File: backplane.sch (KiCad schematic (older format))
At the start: 29 parts, among them J1 I2C, J2 I2C, J3 SER, J4 PWR, J5 PWR, J6 FAN, Q1 Q_NMOS_GSD, Q2 Q_NMOS_GSD, Q3 Q_NMOS_GSD, Q4 Q_NMOS_GSD, U1 Raspberry_Pi_2_3, U2 IC880A-SPI, U3 SHT21, U4 MP1584_MODULE

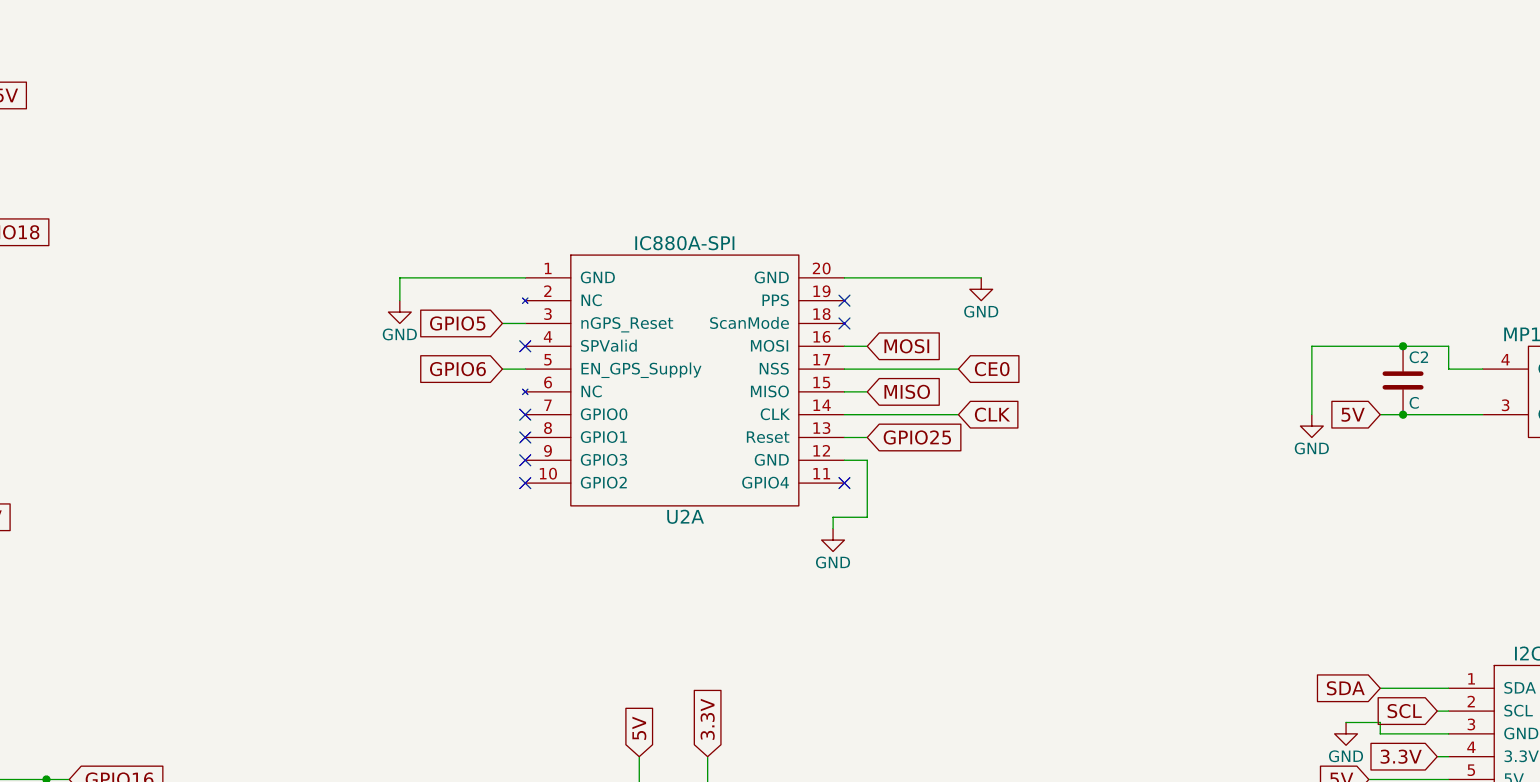
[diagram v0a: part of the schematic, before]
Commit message: Add ADC (refs #14)
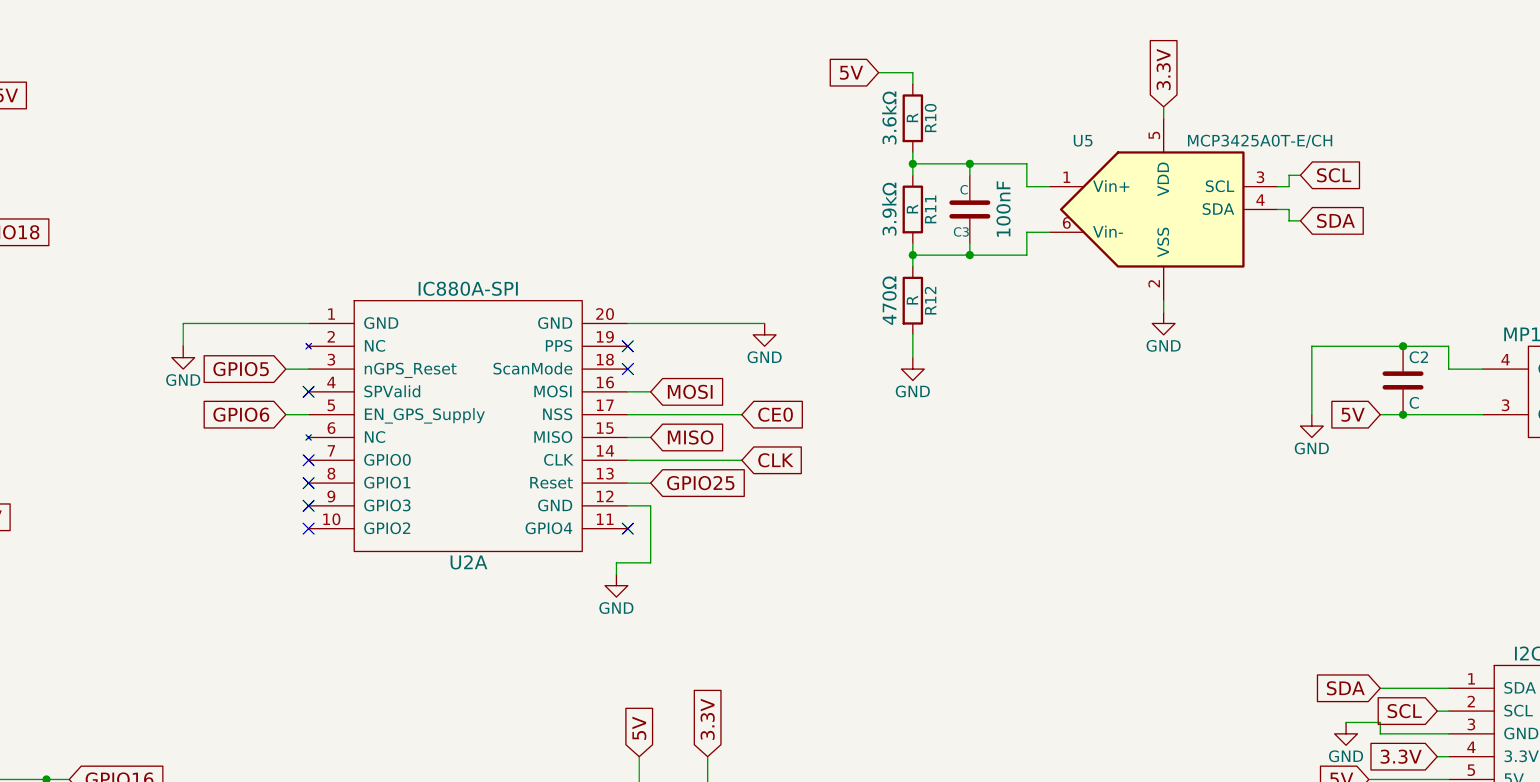
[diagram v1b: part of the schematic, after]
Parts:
- added C3: C, Capacitors_SMD:C_1206, symbol C
- added R10, R11, R12: R, symbol R
- added U5: MCP3425A0T-E/CH, symbol MCP3425A0T-E/CH
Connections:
- net 3.3V: now also U5.5 (VDD)
- net 5V: now also R10.1
- net GND: now also R12.2, U5.2 (VSS)
- net SCL: now also U5.3 (SCL)
- net SDA: now also U5.4 (SDA)
- new net: C3.2, R10.2, R11.1, U5.1 (Vin+)
- new net: C3.1, R11.2, R12.1, U5.6 (Vin-)
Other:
- moved on the sheet: U2A

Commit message: Assign footprints to ADC (refs #14)
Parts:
- R10, R11, R12: footprint (none) -> Resistors_SMD:R_0805_HandSoldering
- U5: footprint (none) -> TO_SOT_Packages_SMD:SOT-23-6_Handsoldering
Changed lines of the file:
@@
 $EndComp
 $Comp
-L GND-RESCUE-backplane #PWR13
+L GND-RESCUE-backplane #PWR01
 U 1 1 58965F26
 P 1650 4000
-F 0 "#PWR13" H 1650 3750 50  0001 C CNN
+F 0 "#PWR01" H 1650 3750 50  0001 C CNN
 F 1 "GND" H 1650 3850 50  0000 C CNN
 F 2 "" H 1650 4000 50  0000 C CNN
@@
 $EndComp
 $Comp
-L GND-RESCUE-backplane #PWR17
+L GND-RESCUE-backplane #PWR02
 U 1 1 58965F7C
 P 850 5000
-F 0 "#PWR17" H 850 4750 50  0001 C CNN
+F 0 "#PWR02" H 850 4750 50  0001 C CNN
 F 1 "GND" H 850 4850 50  0000 C CNN
 F 2 "" H 850 5000 50  0000 C CNN
@@
 $EndComp
 $Comp
-L GND-RESCUE-backplane #PWR15
+L GND-RESCUE-backplane #PWR03
 U 1 1 58965FBA
 P 1250 4500
-F 0 "#PWR15" H 1250 4250 50  0001 C CNN
+F 0 "#PWR03" H 1250 4250 50  0001 C CNN
 F 1 "GND" H 1250 4350 50  0000 C CNN
 F 2 "" H 1250 4500 50  0000 C CNN
@@
 $EndComp
 $Comp
-L GND-RESCUE-backplane #PWR21
+L GND-RESCUE-backplane #PWR04
 U 1 1 5896BA26
 P 4950 6850
-F 0 "#PWR21" H 4950 6600 50  0001 C CNN
+F 0 "#PWR04" H 4950 6600 50  0001 C CNN
 F 1 "GND" H 4950 6700 50  0000 C CNN
 F 2 "" H 4950 6850 50  0000 C CNN
@@
 $EndComp
 $Comp
-L GND-RESCUE-backplane #PWR3
+L GND-RESCUE-backplane #PWR05
 U 1 1 589714DC
 P 5750 1750
-F 0 "#PWR3" H 5750 1500 50  0001 C CNN
+F 0 "#PWR05" H 5750 1500 50  0001 C CNN
 F 1 "GND" H 5750 1600 50  0000 C CNN
 F 2 "" H 5750 1750 50  0000 C CNN
@@
 $EndComp
 $Comp
-L GND-RESCUE-backplane #PWR9
+L GND-RESCUE-backplane #PWR06
 U 1 1 589715AD
 P 5100 2850
-F 0 "#PWR9" H 5100 2600 50  0001 C CNN
+F 0 "#PWR06" H 5100 2600 50  0001 C CNN
 F 1 "GND" H 5100 2700 50  0000 C CNN
 F 2 "" H 5100 2850 50  0000 C CNN
@@
 $EndComp
 $Comp
-L GND-RESCUE-backplane #PWR6
+L GND-RESCUE-backplane #PWR07
 U 1 1 589716C7
 P 3200 1850
-F 0 "#PWR6" H 3200 1600 50  0001 C CNN
+F 0 "#PWR07" H 3200 1600 50  0001 C CNN
 F 1 "GND" H 3200 1700 50  0000 C CNN
 F 2 "" H 3200 1850 50  0000 C CNN
@@
 $EndComp
 $Comp
-L GND #PWR20
+L GND #PWR08
 U 1 1 5898B674
 P 2200 6400
-F 0 "#PWR20" H 2200 6400 30  0001 C CNN
+F 0 "#PWR08" H 2200 6400 30  0001 C CNN
 F 1 "GND" H 2200 6330 30  0001 C CNN
 F 2 "" H 2200 6400 60  0001 C CNN
@@
 F 1 "SHT21" H 9350 5300 60  0000 C CNN
 F 2 "sensirion:SHT21" H 9350 5000 60  0001 C CNN
-F 3 "" H 9350 5000 60  0001 C CNN
+F 3 "https://www.sensirion.com/fileadmin/user_upload/customers/sensirion/Dokumente/2_Humidity_Sensors/Sensirion_Humidity_Sensors_SHT21_Datasheet_V4.pdf" H 9350 5000 60  0001 C CNN
 	1    9350 5000
 	1    0    0    -1
@@
 F 1 "C" H 9356 4415 40  0000 L CNN
 F 2 "Capacitors_SMD:C_1206" H 9388 4350 30  0001 C CNN
-F 3 "https://www.sensirion.com/fileadmin/user_upload/customers/sensirion/Dokumente/2_Humidity_Sensors/Sensirion_Humidity_Sensors_SHT21_Datasheet_V4.pdf" H 9350 4500 60  0001 C CNN
+F 3 "" H 9350 4500 60  0001 C CNN
 F 4 "100nF" V 9200 4500 60  0000 C CNN "C"
 	1    9350 4500
@@
 $EndComp
 $Comp
-L GND #PWR12
+L GND #PWR09
 U 1 1 58A239AE
 P 2200 3950
-F 0 "#PWR12" H 2200 3700 50  0001 C CNN
+F 0 "#PWR09" H 2200 3700 50  0001 C CNN
 F 1 "GND" H 2200 3800 50  0000 C CNN
 F 2 "" H 2200 3950 50  0000 C CNN
@@
 $EndComp
 $Comp
-L GND #PWR14
+L GND #PWR010
 U 1 1 58A23A76
 P 2200 4450
-F 0 "#PWR14" H 2200 4200 50  0001 C CNN
+F 0 "#PWR010" H 2200 4200 50  0001 C CNN
 F 1 "GND" H 2200 4300 50  0000 C CNN
 F 2 "" H 2200 4450 50  0000 C CNN
@@
 $EndComp
 $Comp
-L GND #PWR16
+L GND #PWR011
 U 1 1 58A23B3E
 P 2200 4950
-F 0 "#PWR16" H 2200 4700 50  0001 C CNN
+F 0 "#PWR011" H 2200 4700 50  0001 C CNN
 F 1 "GND" H 2200 4800 50  0000 C CNN
 F 2 "" H 2200 4950 50  0000 C CNN
@@
 $EndComp
 $Comp
-L GND #PWR5
+L GND #PWR012
 U 1 1 58A90AD5
 P 2000 1850
-F 0 "#PWR5" H 2000 1600 50  0001 C CNN
+F 0 "#PWR012" H 2000 1600 50  0001 C CNN
 F 1 "GND" H 2000 1700 50  0000 C CNN
 F 2 "" H 2000 1850 50  0000 C CNN
@@
 5V
 $Comp
-L GND #PWR4
+L GND #PWR013
 U 1 1 58F15EFB
 P 1600 1850
-F 0 "#PWR4" H 1600 1600 50  0001 C CNN
+F 0 "#PWR013" H 1600 1600 50  0001 C CNN
 F 1 "GND" H 1600 1700 50  0000 C CNN
 F 2 "" H 1600 1850 50  0000 C CNN
@@
 $EndComp
 $Comp
-L GND #PWR8
+L GND #PWR014
 U 1 1 58F163DE
 P 8150 2150
-F 0 "#PWR8" H 8150 1900 50  0001 C CNN
+F 0 "#PWR014" H 8150 1900 50  0001 C CNN
 F 1 "GND" H 8150 2000 50  0000 C CNN
 F 2 "" H 8150 2150 50  0000 C CNN
@@
 5V
 $Comp
-L GND #PWR1
+L GND #PWR015
 U 1 1 58F16888
 P 9750 1350
-F 0 "#PWR1" H 9750 1100 50  0001 C CNN
+F 0 "#PWR015" H 9750 1100 50  0001 C CNN
 F 1 "GND" H 9750 1200 50  0000 C CNN
 F 2 "" H 9750 1350 50  0000 C CNN
@@
 GPIO18
 $Comp
-L GND #PWR19
+L GND #PWR016
 U 1 1 58F17ECB
 P 3750 6250
-F 0 "#PWR19" H 3750 6000 50  0001 C CNN
+F 0 "#PWR016" H 3750 6000 50  0001 C CNN
 F 1 "GND" H 3750 6100 50  0000 C CNN
 F 2 "" H 3750 6250 50  0000 C CNN
@@
 5V
 $Comp
-L PWR_FLAG #FLG1
+L PWR_FLAG #FLG017
 U 1 1 58F18E09
 P 3750 6150
-F 0 "#FLG1" H 3750 6245 50  0001 C CNN
+F 0 "#FLG017" H 3750 6245 50  0001 C CNN
 F 1 "PWR_FLAG" H 3750 6330 50  0000 C CNN
 F 2 "" H 3750 6150 50  0000 C CNN
@@
 SDA
 $Comp
-L GND #PWR11
+L GND #PWR018
 U 1 1 58F1F392
 P 9600 3500
-F 0 "#PWR11" H 9600 3250 50  0001 C CNN
+F 0 "#PWR018" H 9600 3250 50  0001 C CNN
 F 1 "GND" H 9600 3350 50  0000 C CNN
 F 2 "" H 9600 3500 50  0000 C CNN
@@
 SDA
 $Comp
-L GND #PWR10
+L GND #PWR019
 U 1 1 58F20596
 P 8300 3500
-F 0 "#PWR10" H 8300 3250 50  0001 C CNN
+F 0 "#PWR019" H 8300 3250 50  0001 C CNN
 F 1 "GND" H 8300 3350 50  0000 C CNN
 F 2 "" H 8300 3500 50  0000 C CNN
@@
 3.3V
 $Comp
-L GND #PWR18
+L GND #PWR020
 U 1 1 58F2395B
 P 10250 5050
-F 0 "#PWR18" H 10250 4800 50  0001 C CNN
+F 0 "#PWR020" H 10250 4800 50  0001 C CNN
 F 1 "GND" H 10250 4900 50  0000 C CNN
 F 2 "" H 10250 5050 50  0000 C CNN
@@
 F 0 "U5" H 7100 1550 50  0000 L CNN
 F 1 "MCP3425A0T-E/CH" H 7600 1550 50  0000 L CNN
-F 2 "" H 7500 1250 50  0000 C CIN
+F 2 "TO_SOT_Packages_SMD:SOT-23-6_Handsoldering" H 7500 1250 50  0001 C CIN
 F 3 "" H 7500 1250 50  0000 C CNN
 	1    7500 1250
@@
 	7500 1650 7500 1700
 $Comp
-L GND #PWR2
+L GND #PWR021
 U 1 1 58F1498B
 P 7500 1700
-F 0 "#PWR2" H 7500 1450 50  0001 C CNN
+F 0 "#PWR021" H 7500 1450 50  0001 C CNN
 F 1 "GND" H 7500 1550 50  0000 C CNN
 F 2 "" H 7500 1700 50  0000 C CNN
@@
 F 0 "R11" V 6480 1250 50  0000 C CNN
 F 1 "R" V 6400 1250 50  0000 C CNN
-F 2 "" V 6330 1250 50  0000 C CNN
+F 2 "Resistors_SMD:R_0805_HandSoldering" V 6330 1250 50  0001 C CNN
 F 3 "" H 6400 1250 50  0000 C CNN
 F 4 "3.9kΩ" V 6300 1250 60  0000 C CNN "R"
@@
 F 0 "R10" V 6480 850 50  0000 C CNN
 F 1 "R" V 6400 850 50  0000 C CNN
-F 2 "" V 6330 850 50  0000 C CNN
+F 2 "Resistors_SMD:R_0805_HandSoldering" V 6330 850 50  0001 C CNN
 F 3 "" H 6400 850 50  0000 C CNN
 F 4 "3.6kΩ" V 6300 850 60  0000 C CNN "R"
@@
 F 0 "R12" V 6480 1650 50  0000 C CNN
 F 1 "R" V 6400 1650 50  0000 C CNN
-F 2 "" V 6330 1650 50  0000 C CNN
+F 2 "Resistors_SMD:R_0805_HandSoldering" V 6330 1650 50  0001 C CNN
 F 3 "" H 6400 1650 50  0000 C CNN
 F 4 "470Ω" V 6300 1650 60  0000 C CNN "R"
@@
 	6400 1800 6400 1900
 $Comp
-L GND #PWR7
+L GND #PWR022
 U 1 1 58F15D89
 P 6400 1900
-F 0 "#PWR7" H 6400 1650 50  0001 C CNN
+F 0 "#PWR022" H 6400 1650 50  0001 C CNN
 F 1 "GND" H 6400 1750 50  0000 C CNN
 F 2 "" H 6400 1900 50  0000 C CNN
@@
 	7000 1350 6900 1350
 Wire Wire Line
-	6900 1450 6900 1350
-Wire Wire Line
-	6400 1450 6900 1450
+	6900 1350 6900 1450
+Wire Wire Line
+	6900 1450 6400 1450
 Connection ~ 6400 1450
 Text GLabel 6250 650  0    60   Input ~ 0
@@
 F 1 "C" H 6656 1165 40  0000 L CNN
 F 2 "Capacitors_SMD:C_1206" H 6688 1100 30  0001 C CNN
-F 3 "https://www.sensirion.com/fileadmin/user_upload/customers/sensirion/Dokumente/2_Humidity_Sensors/Sensirion_Humidity_Sensors_SHT21_Datasheet_V4.pdf" H 6650 1250 60  0001 C CNN
+F 3 "" H 6650 1250 60  0001 C CNN
 F 4 "100nF" V 6500 1250 60  0000 C CNN "C"
 	1    6650 1250

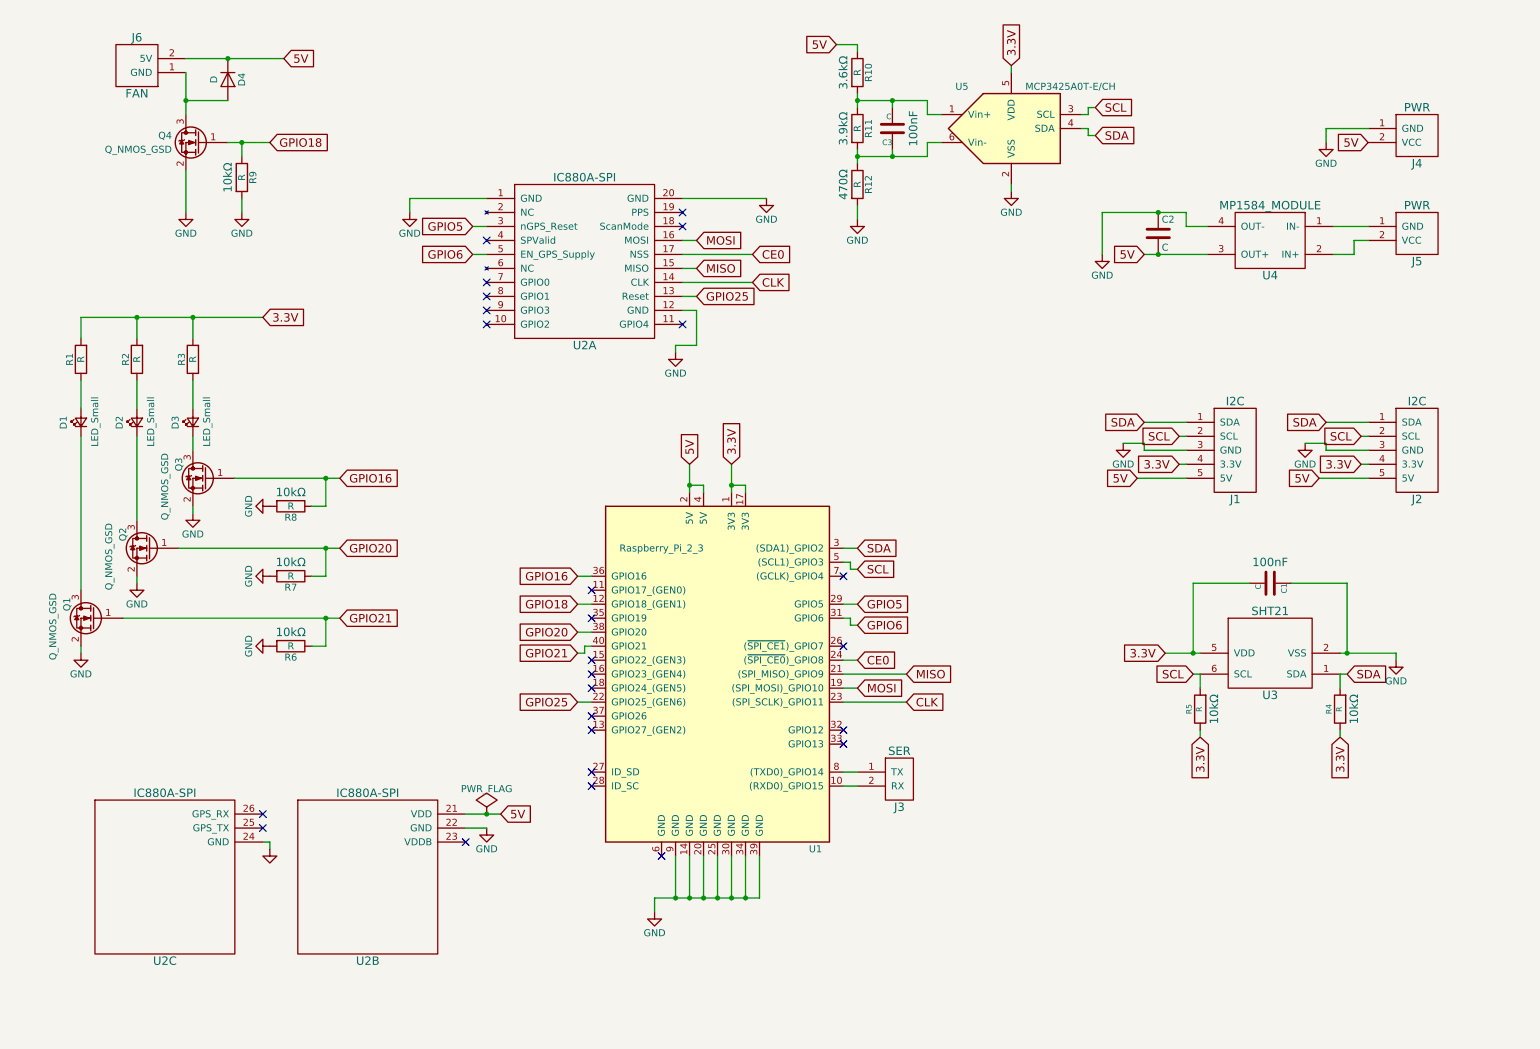
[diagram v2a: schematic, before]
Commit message: Clean up schematics
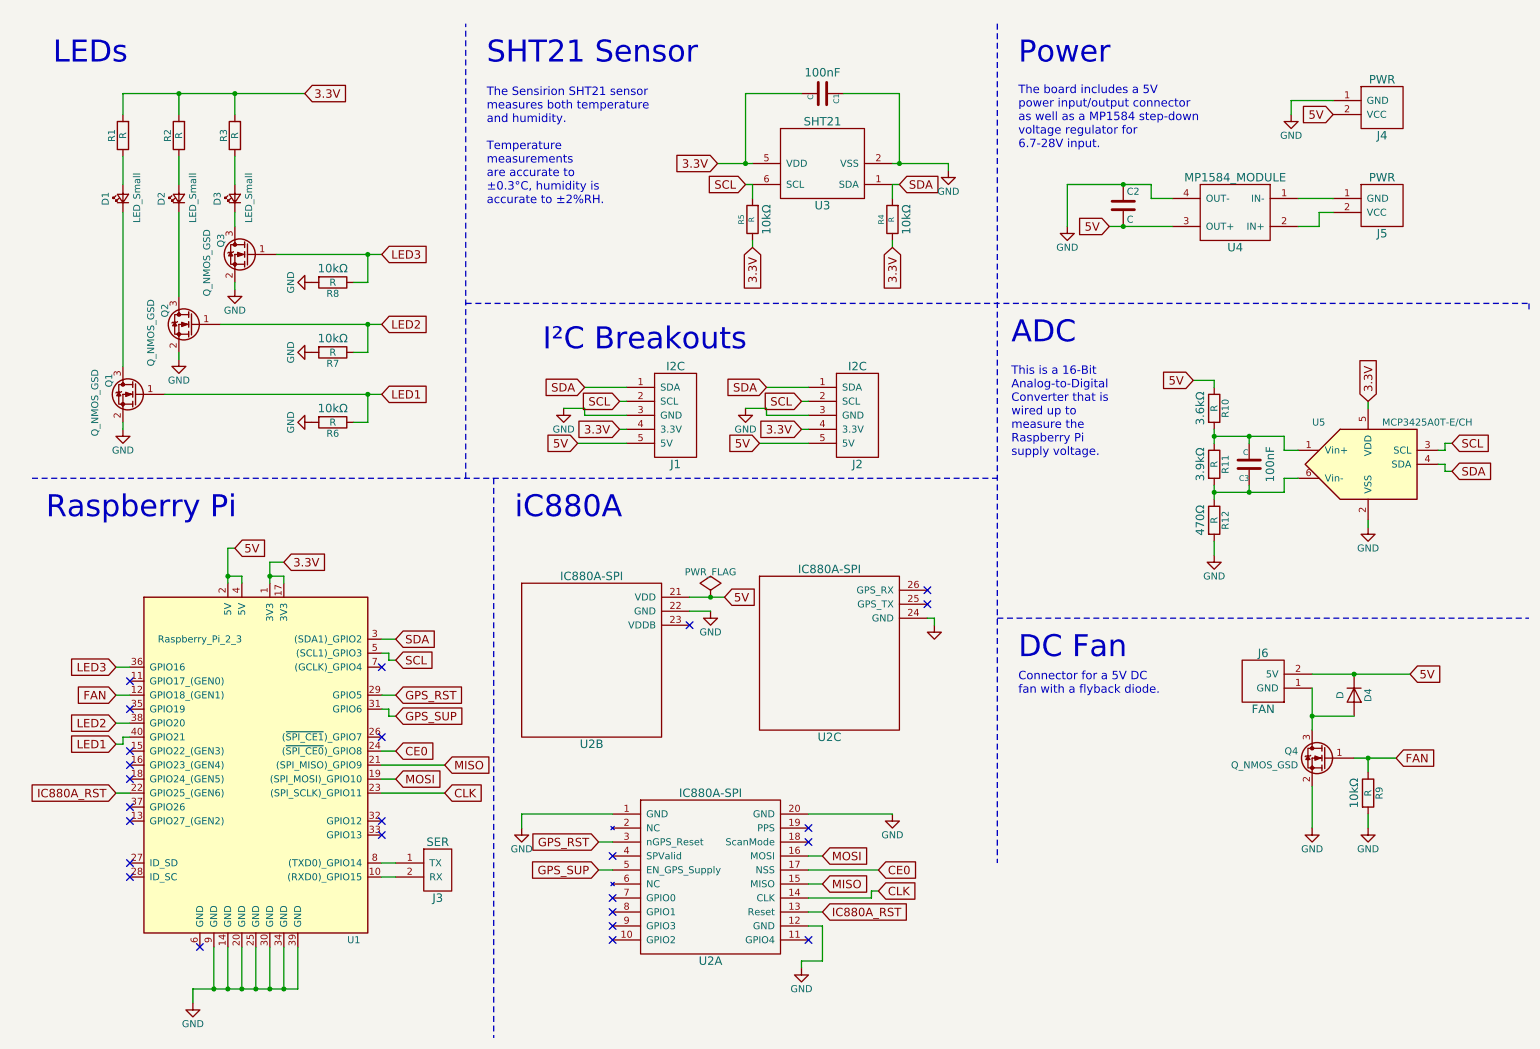
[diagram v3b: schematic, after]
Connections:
- net GPIO16 renamed LED3
- net GPIO18 renamed FAN
- net GPIO20 renamed LED2
- net GPIO21 renamed LED1
- net GPIO25 renamed IC880A_RST
- net GPIO5 renamed GPS_RST
- net GPIO6 renamed GPS_SUP
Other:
- note added: "ADC"
- note added: "Connector for a 5V DC\nfan with a flyback diode."
- note added: "DC Fan"
- note added: "I²C Breakouts"
- note added: "LEDs"
- note added: "Power"
- note added: "Raspberry Pi"
- note added: "SHT21 Sensor"
- note added: "The Sensirion SHT21 sensor\nmeasures both temperature\nand humidity.\n\nTemperature\nmeasurements\nare accurate to\n±0.3°C, humidity is\naccurate to ±2%RH."
- note added: "The board includes a 5V\npower input/output connector\nas well as a MP1584 step-down\nvoltage regulator for\n6.7-28V input."
- note added: "This is a 16-Bit\nAnalog-to-Digital\nConverter that is\nwired up to\nmeasure the\nRaspberry Pi\nsupply voltage."
- note added: "iC880A"
- moved on the sheet: C1, C2, C3, D1, D2, D3, D4, J1, J2, J3, J4, J5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
